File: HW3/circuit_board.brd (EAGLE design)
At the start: 50 x 50 mm, 21 parts

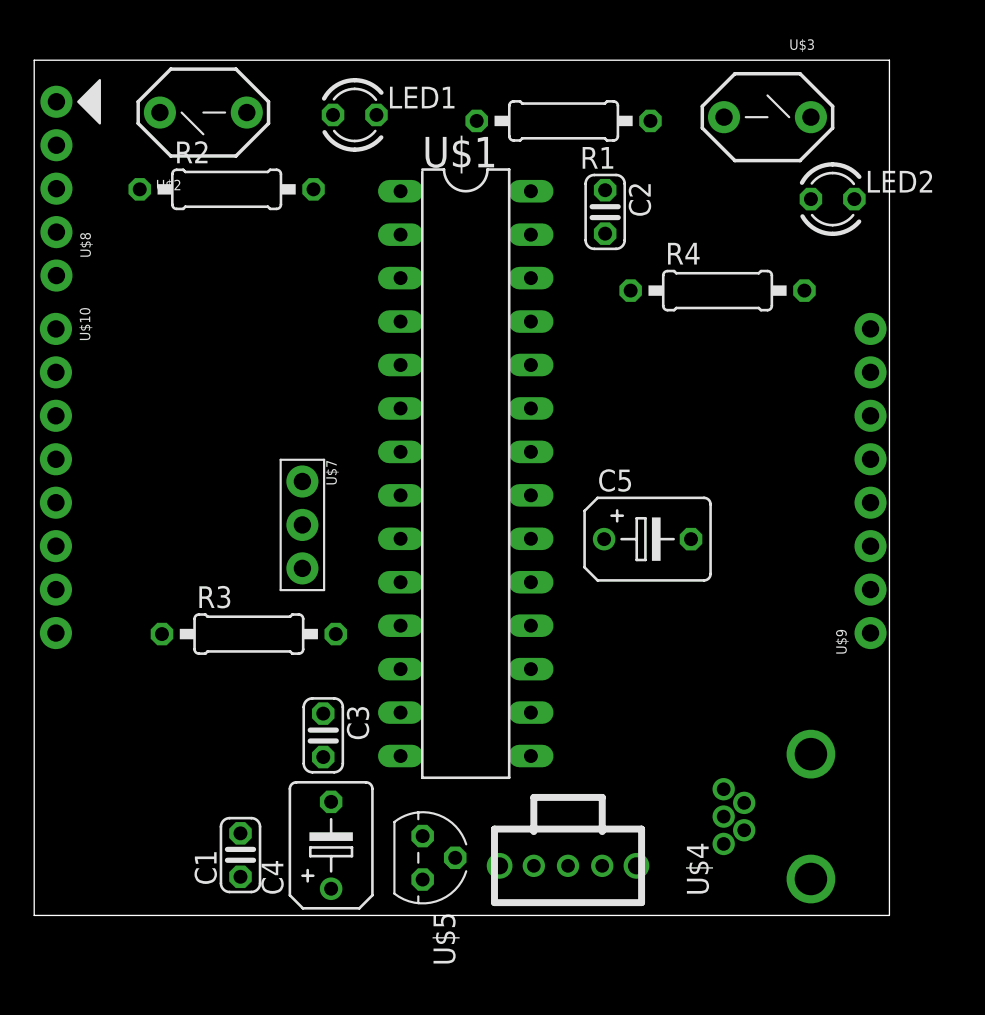
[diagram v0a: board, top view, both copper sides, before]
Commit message: Small changes
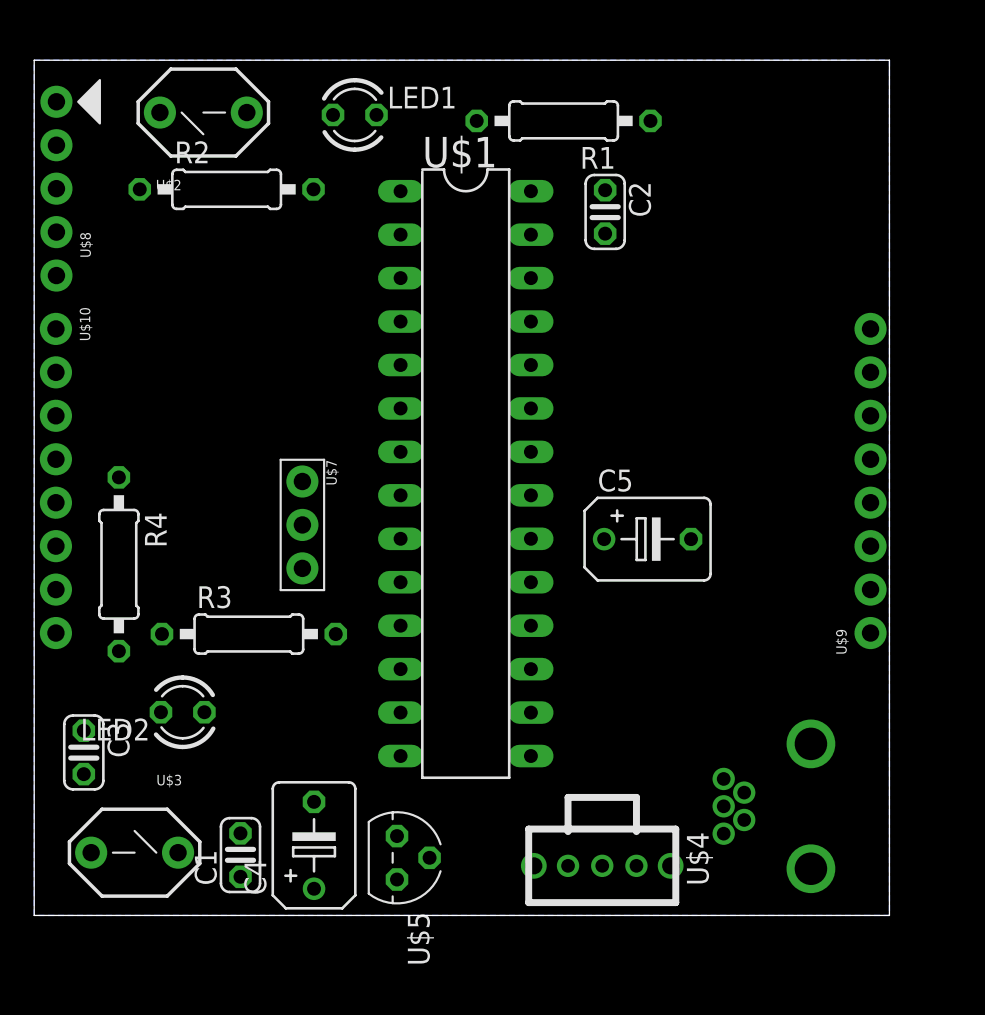
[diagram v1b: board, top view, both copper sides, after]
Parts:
- moved U$3 56.7 mm to (3.33, 3.67)
- moved LED2 48.4 mm to (8.68, 11.9), turned to 180 degrees
- moved R4 38.5 mm to (4.95, 20.5), turned to 270 degrees
- moved C3 14.0 mm to (2.90, 9.53)
- moved U$6 2.00 mm to (33.2, 2.90)
- moved U$5 1.50 mm to (21.2, 3.37)
- moved C4 1.00 mm to (16.4, 4.10)
- moved U$4 0.60 mm to (45.4, 6.38)
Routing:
- added copper zone on layer 16, net GND
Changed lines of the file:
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@@
 <element name="C1" library="resistor" library_urn="urn:adsk.eagle:library:348" package="C025-024X044" package3d_urn="urn:adsk.eagle:package:26149/1" value="" x="12.06" y="3.53" rot="R90"/>
 <element name="C2" library="resistor" library_urn="urn:adsk.eagle:library:348" package="C025-024X044" package3d_urn="urn:adsk.eagle:package:26149/1" value="" x="33.38" y="41.13" rot="R270"/>
-<element name="C3" library="resistor" library_urn="urn:adsk.eagle:library:348" package="C025-024X044" package3d_urn="urn:adsk.eagle:package:26149/1" value="" x="16.9" y="10.53" rot="R270"/>
-<element name="C4" library="resistor" library_urn="urn:adsk.eagle:library:348" package="B45181B" package3d_urn="urn:adsk.eagle:package:25794/1" value="" x="17.36" y="4.1" rot="R90"/>
+<element name="C3" library="resistor" library_urn="urn:adsk.eagle:library:348" package="C025-024X044" package3d_urn="urn:adsk.eagle:package:26149/1" value="" x="2.9" y="9.53" rot="R270"/>
+<element name="C4" library="resistor" library_urn="urn:adsk.eagle:library:348" package="B45181B" package3d_urn="urn:adsk.eagle:package:25794/1" value="" x="16.36" y="4.1" rot="R90"/>
 <element name="C5" library="resistor" library_urn="urn:adsk.eagle:library:348" package="B45181B" package3d_urn="urn:adsk.eagle:package:25794/1" value="" x="35.86" y="22"/>
 <element name="LED1" library="led" library_urn="urn:adsk.eagle:library:259" package="LED3MM" package3d_urn="urn:adsk.eagle:package:15797/1" value="" x="18.74" y="46.8"/>
-<element name="LED2" library="led" library_urn="urn:adsk.eagle:library:259" package="LED3MM" package3d_urn="urn:adsk.eagle:package:15797/1" value="" x="46.68" y="41.88"/>
+<element name="LED2" library="led" library_urn="urn:adsk.eagle:library:259" package="LED3MM" package3d_urn="urn:adsk.eagle:package:15797/1" value="" x="8.68" y="11.88" rot="R180"/>
 <element name="R1" library="resistor" library_urn="urn:adsk.eagle:library:348" package="0207/10" package3d_urn="urn:adsk.eagle:package:25939/1" value="" x="30.95" y="46.45" rot="R180"/>
 <element name="R2" library="resistor" library_urn="urn:adsk.eagle:library:348" package="0207/10" package3d_urn="urn:adsk.eagle:package:25939/1" value="" x="11.25" y="42.45"/>
 <element name="R3" library="resistor" library_urn="urn:adsk.eagle:library:348" package="0207/10" package3d_urn="urn:adsk.eagle:package:25939/1" value="" x="12.55" y="16.45"/>
-<element name="R4" library="resistor" library_urn="urn:adsk.eagle:library:348" package="0207/10" package3d_urn="urn:adsk.eagle:package:25939/1" value="" x="39.95" y="36.53"/>
+<element name="R4" library="resistor" library_urn="urn:adsk.eagle:library:348" package="0207/10" package3d_urn="urn:adsk.eagle:package:25939/1" value="" x="4.95" y="20.53" rot="R270"/>
 <element name="U$1" library="pic32" package="DIL28-3" value="PIC32MX" x="25.23" y="25.83" rot="R270"/>
 <element name="U$10" library="connectior-8pin-holes" package="1X08" value="CONNECTOR_8PIN-HOLES" x="1.27" y="34.29" rot="R270"/>
 <element name="U$2" library="PUSH_BUTTON" package="1X03" value="PUSH_BUTTON_SPST-NO" x="12.43" y="46.94" rot="R180"/>
-<element name="U$3" library="PUSH_BUTTON" package="1X03" value="PUSH_BUTTON_SPST-NO" x="40.33" y="46.67"/>
-<element name="U$4" library="usb_conn" package="USB-MB-H" value="USB_MINI" x="45.41" y="5.78" rot="R180"/>
-<element name="U$5" library="V_REG" package="TO92" value="MCP1072" x="22.71" y="3.37" rot="R270"/>
-<element name="U$6" library="SLIDE_SWITCH" package="SLIDE_SW" value="SLIDE_SWITCH" x="31.21" y="2.9"/>
+<element name="U$3" library="PUSH_BUTTON" package="1X03" value="PUSH_BUTTON_SPST-NO" x="3.33" y="3.67"/>
+<element name="U$4" library="usb_conn" package="USB-MB-H" value="USB_MINI" x="45.41" y="6.38" rot="R180"/>
+<element name="U$5" library="V_REG" package="TO92" value="MCP1072" x="21.21" y="3.37" rot="R270"/>
+<element name="U$6" library="SLIDE_SWITCH" package="SLIDE_SW" value="SLIDE_SWITCH" x="33.21" y="2.9"/>
 <element name="U$7" library="OSC" package="1X03" value="OSC" x="15.68" y="25.37" rot="R270"/>
 <element name="U$8" library="pickit" package="1X05" value="PICKIT" x="1.3" y="47.57" rot="R270"/>
@@
 <wire x1="29.04" y1="29.64" x2="29.04" y2="42.34" width="0" layer="19" extent="1-1"/>
 <wire x1="21.42" y1="11.86" x2="29.04" y2="29.64" width="0" layer="19" extent="1-1"/>
-<wire x1="16.9" y1="11.8" x2="21.42" y2="11.86" width="0" layer="19" extent="1-1"/>
-<wire x1="17.36" y1="1.56" x2="16.9" y2="11.8" width="0" layer="19" extent="1-1"/>
-<wire x1="22.71" y1="2.1" x2="17.36" y2="1.56" width="0" layer="19" extent="1-1"/>
-<wire x1="7.47" y1="16.45" x2="16.9" y2="11.8" width="0" layer="19" extent="1-1"/>
+<wire x1="21.21" y1="2.1" x2="21.42" y2="11.86" width="0" layer="19" extent="1-1"/>
+<wire x1="16.36" y1="1.56" x2="21.21" y2="2.1" width="0" layer="19" extent="1-1"/>
+<wire x1="7.47" y1="16.45" x2="21.42" y2="11.86" width="0" layer="19" extent="1-1"/>
 <wire x1="1.27" y1="19.05" x2="7.47" y2="16.45" width="0" layer="19" extent="1-1"/>
+<wire x1="2.9" y1="10.8" x2="7.47" y2="16.45" width="0" layer="19" extent="1-1"/>
 </signal>
 <signal name="N$1">
@@
 <contactref element="U$10" pad="8"/>
 <contactref element="U$1" pad="8"/>
-<wire x1="33.38" y1="39.86" x2="40.33" y2="46.67" width="0" layer="19" extent="1-1"/>
-<wire x1="34.87" y1="36.53" x2="33.38" y2="39.86" width="0" layer="19" extent="1-1"/>
-<wire x1="29.04" y1="39.8" x2="33.38" y2="39.86" width="0" layer="19" extent="1-1"/>
-<wire x1="25.87" y1="46.45" x2="29.04" y2="39.8" width="0" layer="19" extent="1-1"/>
-<wire x1="38.4" y1="22" x2="34.87" y2="36.53" width="0" layer="19" extent="1-1"/>
-<wire x1="29.04" y1="19.48" x2="38.4" y2="22" width="0" layer="19" extent="1-1"/>
-<wire x1="21.42" y1="24.56" x2="29.04" y2="19.48" width="0" layer="19" extent="1-1"/>
-<wire x1="15.68" y1="22.83" x2="21.42" y2="24.56" width="0" layer="19" extent="1-1"/>
-<wire x1="48.895" y1="16.51" x2="38.4" y2="22" width="0" layer="19" extent="1-1"/>
-<wire x1="40.31" y1="7.38" x2="48.895" y2="16.51" width="0" layer="19" extent="1-1"/>
-<wire x1="16.9" y1="9.26" x2="15.68" y2="22.83" width="0" layer="19" extent="1-1"/>
-<wire x1="17.36" y1="6.64" x2="16.9" y2="9.26" width="0" layer="19" extent="1-1"/>
-<wire x1="12.06" y1="4.8" x2="17.36" y2="6.64" width="0" layer="19" extent="1-1"/>
-<wire x1="22.71" y1="4.64" x2="17.36" y2="6.64" width="0" layer="19" extent="1-1"/>
-<wire x1="1.27" y1="16.51" x2="15.68" y2="22.83" width="0" layer="19" extent="1-1"/>
-<wire x1="7.35" y1="46.94" x2="25.87" y2="46.45" width="0" layer="19" extent="1-1"/>
-<wire x1="1.3" y1="42.49" x2="7.35" y2="46.94" width="0" layer="19" extent="1-1"/>
+<polygon width="0.1524" layer="16" isolate="0.3048">
+<vertex x="0" y="50"/>
+<vertex x="50" y="50"/>
+<vertex x="50" y="0"/>
+<vertex x="0" y="0"/>
+</polygon>
 </signal>
 <signal name="N$2">
 <contactref element="R4" pad="2"/>
 <contactref element="LED2" pad="K"/>
-<wire x1="45.03" y1="36.53" x2="47.95" y2="41.88" width="0" layer="19" extent="1-1"/>
+<wire x1="7.41" y1="11.88" x2="4.95" y2="15.45" width="0" layer="19" extent="1-1"/>
 </signal>
 <signal name="N$3">
@@
 <contactref element="U$6" pad="2"/>
 <contactref element="U$9" pad="2"/>
-<wire x1="40.31" y1="4.18" x2="48.895" y2="19.05" width="0" layer="19" extent="1-1"/>
-<wire x1="31.21" y1="2.9" x2="40.31" y2="4.18" width="0" layer="19" extent="1-1"/>
-<wire x1="29.04" y1="9.32" x2="31.21" y2="2.9" width="0" layer="19" extent="1-1"/>
+<wire x1="40.31" y1="4.78" x2="48.895" y2="19.05" width="0" layer="19" extent="1-1"/>
+<wire x1="33.21" y1="2.9" x2="40.31" y2="4.78" width="0" layer="19" extent="1-1"/>
+<wire x1="29.04" y1="9.32" x2="33.21" y2="2.9" width="0" layer="19" extent="1-1"/>
 </signal>
 <signal name="N$6">
 <contactref element="U$4" pad="D+"/>
 <contactref element="U$1" pad="21"/>
-<wire x1="40.31" y1="5.78" x2="29.04" y2="24.56" width="0" layer="19" extent="1-1"/>
+<wire x1="40.31" y1="6.38" x2="29.04" y2="24.56" width="0" layer="19" extent="1-1"/>
 </signal>
 <signal name="N$7">
 <contactref element="U$4" pad="D-"/>
 <contactref element="U$1" pad="22"/>
-<wire x1="41.51" y1="4.98" x2="29.04" y2="27.1" width="0" layer="19" extent="1-1"/>
+<wire x1="41.51" y1="5.58" x2="29.04" y2="27.1" width="0" layer="19" extent="1-1"/>
 </signal>
 <signal name="N$8">
@@
 <contactref element="U$5" pad="2"/>
 <contactref element="U$6" pad="1"/>
-<wire x1="24.615" y1="3.37" x2="29.21" y2="2.9" width="0" layer="19" extent="1-1"/>
-<wire x1="12.06" y1="2.26" x2="24.615" y2="3.37" width="0" layer="19" extent="1-1"/>
+<wire x1="23.115" y1="3.37" x2="31.21" y2="2.9" width="0" layer="19" extent="1-1"/>
+<wire x1="12.06" y1="2.26" x2="23.115" y2="3.37" width="0" layer="19" extent="1-1"/>
 </signal>
 <signal name="N$9">
@@
 <contactref element="U$1" pad="11"/>
 <contactref element="U$3" pad="2"/>
-<wire x1="21.42" y1="16.94" x2="45.41" y2="46.67" width="0" layer="19" extent="1-1"/>
 <wire x1="17.63" y1="16.45" x2="21.42" y2="16.94" width="0" layer="19" extent="1-1"/>
+<wire x1="8.41" y1="3.67" x2="17.63" y2="16.45" width="0" layer="19" extent="1-1"/>
 <wire x1="1.27" y1="24.13" x2="17.63" y2="16.45" width="0" layer="19" extent="1-1"/>
 </signal>
@@
 <contactref element="LED2" pad="A"/>
 <contactref element="U$1" pad="12"/>
-<wire x1="21.42" y1="14.4" x2="45.41" y2="41.88" width="0" layer="19" extent="1-1"/>
-<wire x1="1.27" y1="21.59" x2="21.42" y2="14.4" width="0" layer="19" extent="1-1"/>
+<wire x1="9.95" y1="11.88" x2="21.42" y2="14.4" width="0" layer="19" extent="1-1"/>
+<wire x1="1.27" y1="21.59" x2="9.95" y2="11.88" width="0" layer="19" extent="1-1"/>
 </signal>
 <signal name="RB15">
@@
 <contactref element="U$1" pad="14"/>
 <contactref element="U$4" pad="ID"/>
-<wire x1="21.42" y1="9.32" x2="41.51" y2="6.58" width="0" layer="19" extent="1-1"/>
+<wire x1="21.42" y1="9.32" x2="41.51" y2="7.18" width="0" layer="19" extent="1-1"/>
 </signal>
 </signals>
